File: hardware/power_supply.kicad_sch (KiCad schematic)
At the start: 34 parts, among them U2 AP63203WU, U4 TPS62A04ADRL, U5 PLMR51635XDDCR

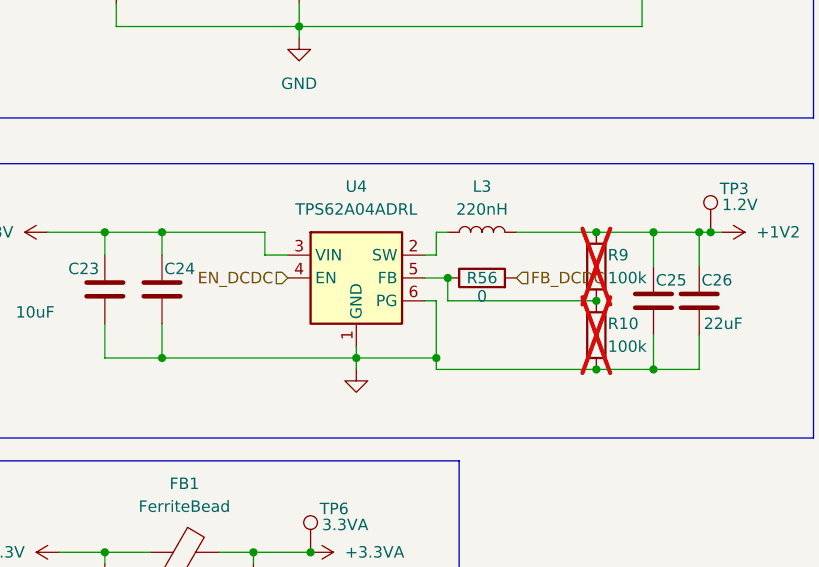
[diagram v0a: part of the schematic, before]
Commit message: 🔥 Redo the PCB
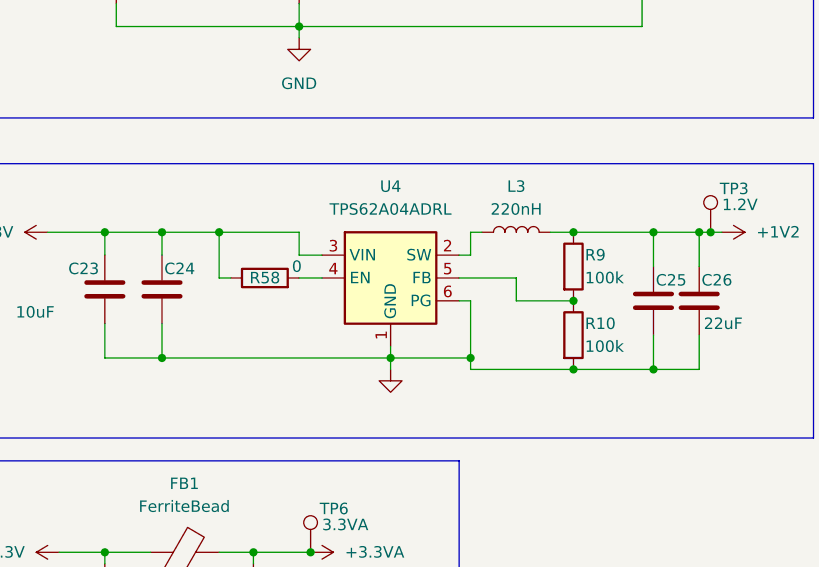
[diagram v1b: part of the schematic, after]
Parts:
- removed R56: 0, PCM_Resistor_SMD_AKL:R_0402_1005Metric, symbol Device:R
- added R58: 0, PCM_Resistor_SMD_AKL:R_0402_1005Metric, symbol Device:R
- R10, R9: now fitted
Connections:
- net +3.3V: now also R58.1
- net EN_DCDC: no longer names the net of U4.4 (EN)
- net EN_DCDC: now also R58.2
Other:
- moved on the sheet: L3, U4
